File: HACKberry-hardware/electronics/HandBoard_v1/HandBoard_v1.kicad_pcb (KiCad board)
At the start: 2 copper layers, 60.8 x 54.8 mm, 10 parts, among them CON1 BARREL_JACK_MJ179PH, SW1 SW_PUSH_SKRGAQD010, SW2 SW_PUSH_SKRGAQD010, SW3 SW_PUSH_SKRGAQD010, SW4 SWITCH_SS-12SDP2, U2 3-CONDUCTOR_MINIATUIRE_JACK_M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, U3 Arduino_Micro, U5 Servo_Motor_MG90S, U6 Servo_Motor_S03N, U7 Servo_Motor_MG90S

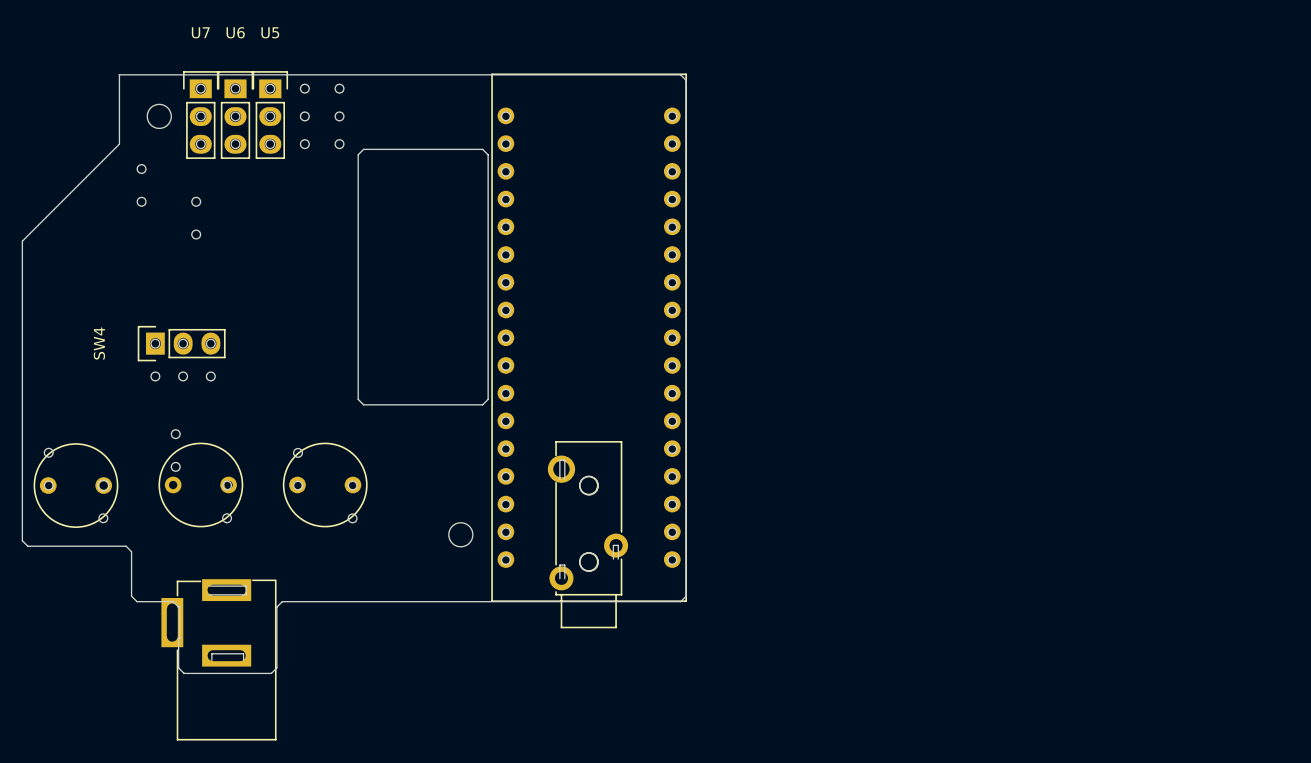
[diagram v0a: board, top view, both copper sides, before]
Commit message: made the garber data of the HandBoard_v1
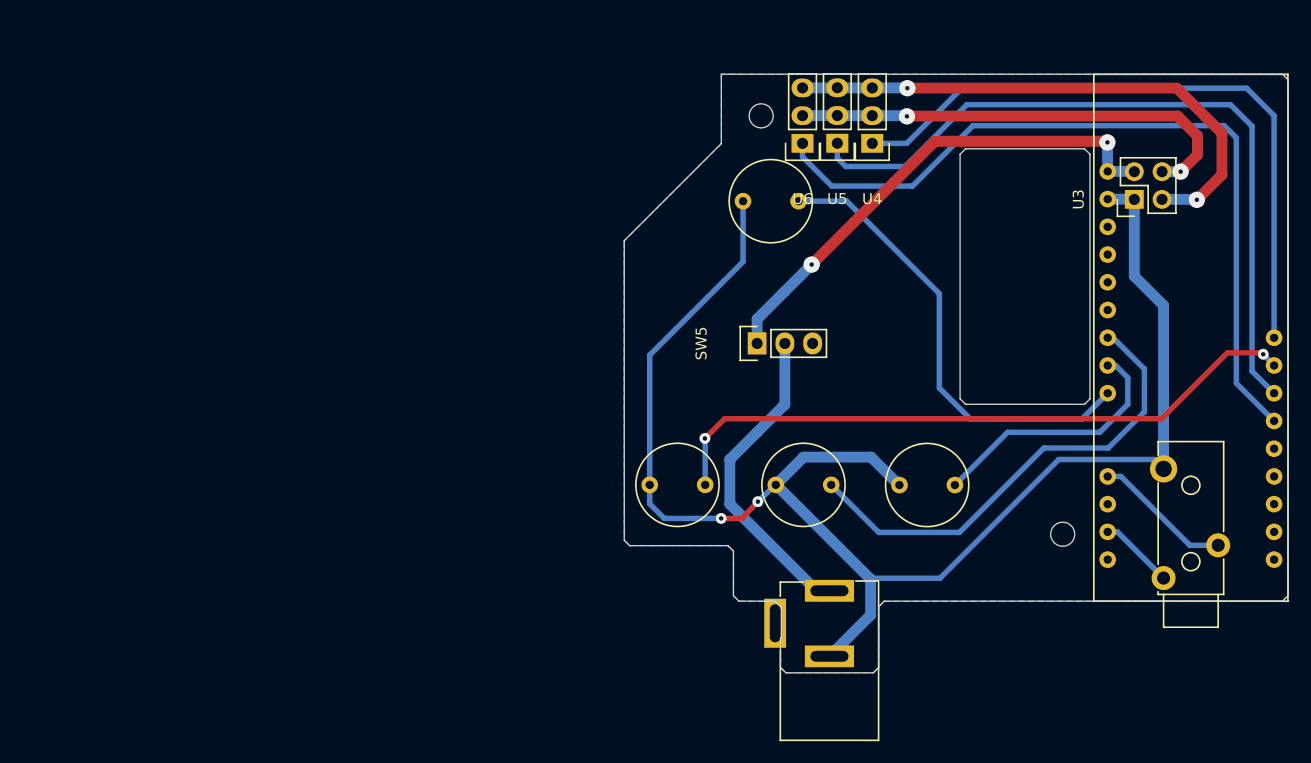
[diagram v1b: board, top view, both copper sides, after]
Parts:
- removed SW1, SW2, SW3: SW_PUSH_SKRGAQD010, HACKberry_v1:SKRGAQ0010
- removed SW4: SWITCH_SS-12SDP2, Pin_Headers:Pin_Header_Straight_1x03
- removed U7: Servo_Motor_MG90S, Pin_Headers:Pin_Header_Straight_1x03
- added SW1:MAX1: SW_PUSH_SKRGAQD010, HACKberry_v1:SKRGAQ0010, F.Cu at (101.5, 118.5)
- added SW2:MIN1: SW_PUSH_SKRGAQD010, HACKberry_v1:SKRGAQ0010, F.Cu at (113.0, 118.5)
- added SW3:Thumb1: SW_PUSH_SKRGAQD010, HACKberry_v1:SKRGAQ0010, F.Cu at (124.3, 118.5)
- added SW4:Middle1: SW_PUSH_SKRGAQD010, HACKberry_v1:SKRGAQ0010, F.Cu at (110.0, 92.5)
- added SW5: SWITCH_SS-12SDP2, Pin_Headers:Pin_Header_Straight_1x03, F.Cu at (108.8, 105.5)
- added U1: 3-CONDUCTOR_MINIATUIRE_JACK_MJ-4535-3, HACKberry_v1:MINIATURE_JACK_MJ-4535-3, F.Cu at (148.5, 125.5)
- added U4: Servo_Motor_S03N, Pin_Headers:Pin_Header_Straight_1x03, F.Cu at (119.3, 87.2)
- U2: value 3-CONDUCTOR_MINIATUIRE_JACK_MJ-4535-3 -> Arduino_Micro; footprint HACKberry_v1:MINIATURE_JACK_MJ-4535-3 -> HACKberry_v1:Arduino_Micro
- U3: value Arduino_Micro -> Seed_Studio_Adjustable_DC/DC_Power_Converter_(1.25V_-_35V/3A); footprint HACKberry_v1:Arduino_Micro -> Pin_Headers:Pin_Header_Straight_2x02
- U6: value Servo_Motor_S03N -> Servo_Motor_MG90S
- moved U2 58.9 mm to (148.5, 105.0), turned to 0 degrees
- moved CON1 55.2 mm to (115.4, 141.9)
- moved U6 52.2 mm to (112.9, 87.2), turned to 180 degrees
- moved U5 52.2 mm to (116.1, 87.2), turned to 180 degrees
- moved U3 51.5 mm to (143.3, 92.3), turned to 90 degrees
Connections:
- U3 pad 2: Net-(U3-Pad2) -> Net-(CON1-Pad3)
- U5 pad 1: Net-(U3-Pad3) -> Net-(U2-Pad5)
- U5 pad 2: Net-(U4-Pad4) -> Net-(U3-Pad4)
- U5 pad 3: Net-(U4-Pad3) -> Net-(U3-Pad3)
- U6 pad 1: Net-(U3-Pad5) -> Net-(U2-Pad6)
- U6 pad 2: Net-(U4-Pad4) -> Net-(U3-Pad4)
- U6 pad 3: Net-(U4-Pad3) -> Net-(U3-Pad3)
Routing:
- net Net-(CON1-Pad3): track 0.00 -> 137.2 mm, vias 0 -> 2
- net Net-(U2-Pad6): track 0.00 -> 72.2 mm
- net Net-(U2-Pad5): track 0.00 -> 68.1 mm
- net Net-(U2-Pad3): track 0.00 -> 60.3 mm
- net Net-(SW1:MAX1-Pad2): track 0.00 -> 60.1 mm, vias 0 -> 2
- net Net-(U3-Pad3): track 0.00 -> 50.4 mm, vias 0 -> 2
- net Net-(SW5-Pad1): track 0.00 -> 46.5 mm, vias 0 -> 2
- net Net-(SW2:MIN1-Pad2): track 0.00 -> 43.5 mm
- net Net-(SW4:Middle1-Pad2): track 0.00 -> 42.6 mm
- net Net-(U3-Pad4): track 0.00 -> 42.6 mm, vias 0 -> 2
- net Net-(CON1-Pad1): track 0.00 -> 28.8 mm
- net Net-(SW3:Thumb1-Pad2): track 0.00 -> 23.6 mm
- net Net-(U1-Pad4): track 0.00 -> 12.7 mm
- net Net-(U1-Pad2): track 0.00 -> 6.87 mm
- net Net-(U2-PadGND): track 0.00 -> 2.41 mm
- added copper zone on B.Cu, net Net-(CON1-Pad3)
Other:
- outline, holes or cut-outs redrawn
- net class Custom01 added: clearance 0.2, trace_width 1, via_dia 2, via_drill 0.4
- net class Default: trace_width 0.25 -> 0.5; via_dia 0.6 -> 1
